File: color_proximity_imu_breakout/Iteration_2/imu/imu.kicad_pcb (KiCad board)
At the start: 2 copper layers, 12.6 x 16.5 mm, 11 parts, among them J4 Conn_01x05, U6 ICM-20602

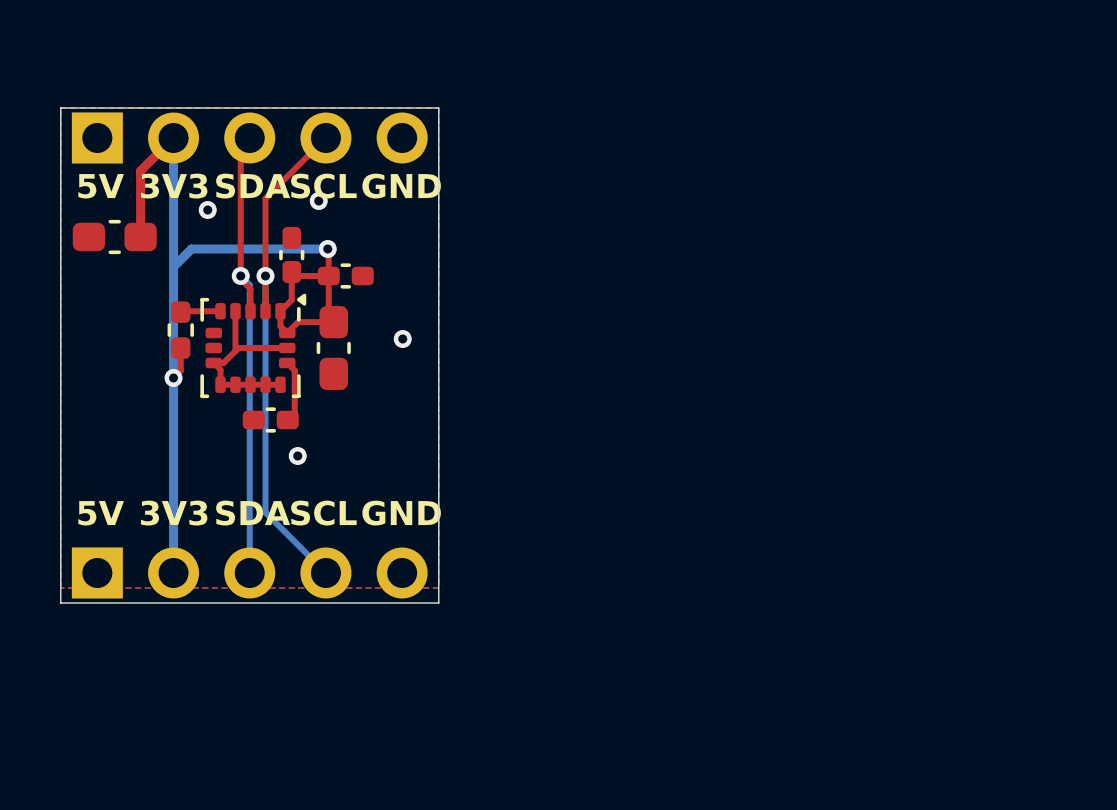
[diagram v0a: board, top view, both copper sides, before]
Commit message: imu updated iteration 2
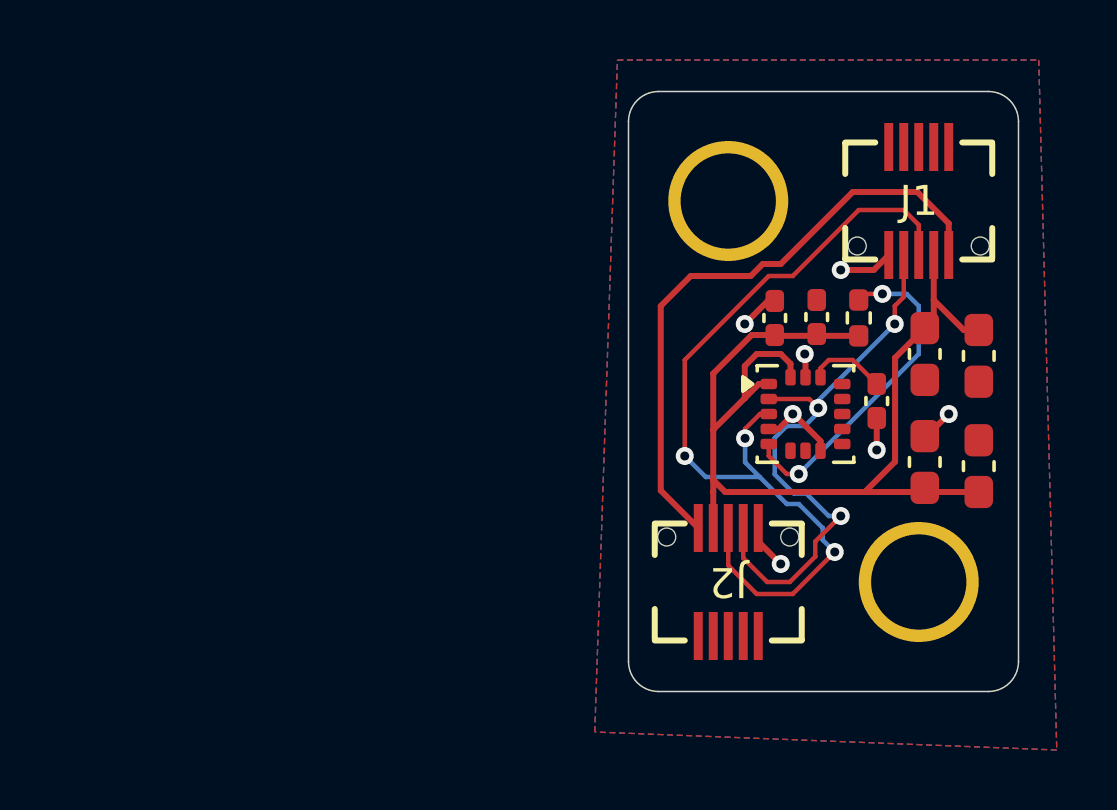
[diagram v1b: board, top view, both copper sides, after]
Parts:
- removed the G*** at (124.4, 134.3)
- removed J4 (x2): Conn_01x05, Connector_PinHeader_2.54mm:PinHeader_1x05_P2.54mm_Vertical
- added ?: , , F.Cu at (142.4, 128.3)
- added ?: , , F.Cu at (148.8, 141.0)
- added C1: 10u, Capacitor_SMD:C_0603_1608Metric_Pad1.08x0.95mm_HandSolder, F.Cu at (149.0, 133.4)
- added C2: 10u, Capacitor_SMD:C_0603_1608Metric_Pad1.08x0.95mm_HandSolder, F.Cu at (150.8, 133.5)
- added G***: LOGO, pcb_footprints:vexu_ghost, B.Cu at (141.8, 138.2)
- added G***: LOGO, pcb_footprints:ras, B.Cu at (144.2, 142.2)
- added J1: Conn_01x10, pcb_footprints:GT-B0502MSV27-10S1101, F.Cu at (148.8, 128.3)
- added J2: Conn_01x10, pcb_footprints:GT-B0502MSV27-10S1101, F.Cu at (142.4, 141.0)
- moved C13 28.0 mm to (149.0, 137.0), turned to 90 degrees
- moved R19 22.6 mm to (146.8, 132.2)
- moved C8 21.9 mm to (150.8, 137.1), turned to 90 degrees
- moved C10 20.2 mm to (147.4, 135.0), turned to -90 degrees
- moved U6 18.6 mm to (145.0, 135.4), turned to 0 degrees
- moved C7 17.6 mm to (145.4, 132.2)
- moved G*** 16.1 mm to (146.6, 136.8)
- moved C9 14.4 mm to (144.0, 132.2), turned to 90 degrees
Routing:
- net +5V: track 0.02 -> 20.6 mm
- net /sda: track 16.3 -> 29.4 mm, vias 1 -> 3
- net Net-(U6-~{CS}): track 1.34 -> 11.4 mm, vias 0 -> 2
- net +3.3V: track 33.0 -> 37.3 mm, vias 2 -> 0
- net GND: track 6.80 -> 10.3 mm, vias 4 -> 7
- net /scl: track 17.3 -> 19.8 mm, vias 1 -> 3
- net Net-(U6-REGOUT): track 2.10 -> 2.62 mm
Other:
- board size 12.6 x 16.5 mm -> 13 x 20 mm
- board text added: "Designed By Gengwen Li Trung Le"
- board text removed: "3V3"
- board text removed: "5V"
- board text removed: "Designed By Gengwen Li"
- board text removed: "GND"
- board text removed: "SCL"
- board text removed: "SDA"
